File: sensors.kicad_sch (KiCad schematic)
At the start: 17 parts, among them Q2 TEMT6000X01, U6 BME280, U7 MAX4466EXK

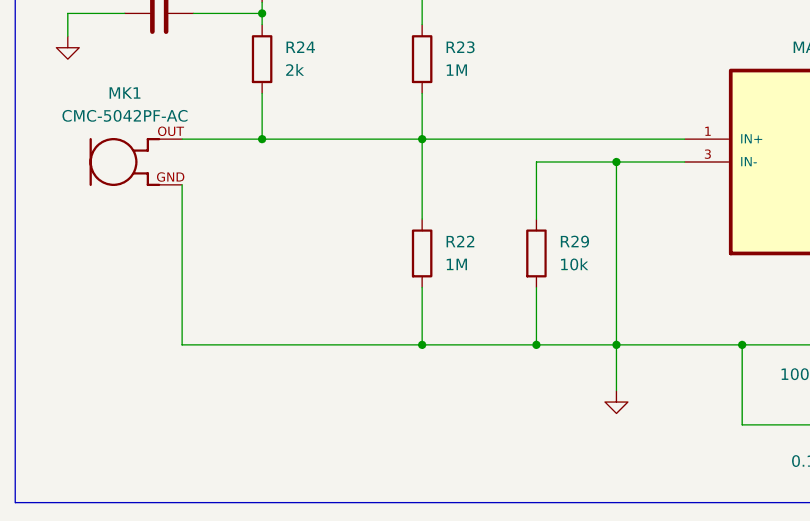
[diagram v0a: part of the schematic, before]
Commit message: wip layout 1
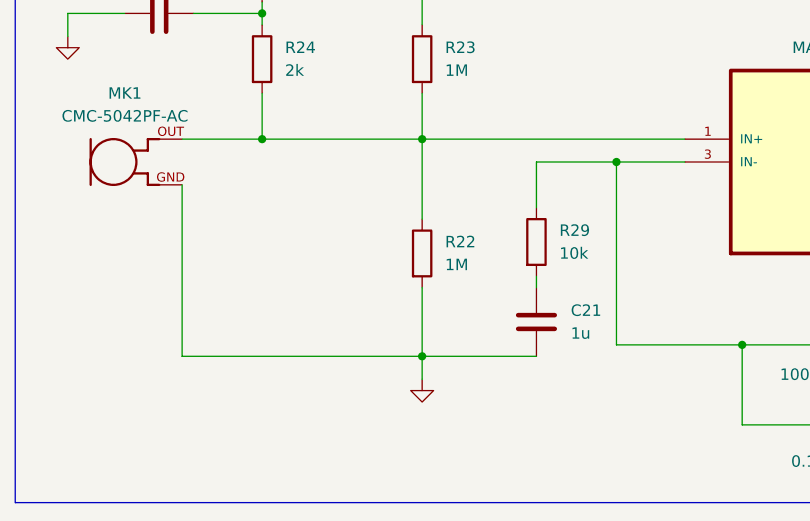
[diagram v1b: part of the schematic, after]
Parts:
- added C21: 1u, Capacitor_SMD:C_0805_2012Metric, symbol Device:C
- MK1: footprint CMC-5042PF-AC:CUI_CMC-5042PF-AC -> esp32 footprints:CUI_CMC-5042PF-AC
- Q2: footprint TEMT6000X01:TRANS_TEMT6000X01 -> esp32 footprints:TRANS_TEMT6000X01
- U6: footprint BME280:PSON65P250X250X100-8N -> esp32 footprints:PSON65P250X250X100-8N
- U7: footprint MAX4466EXK:SOT65P210X110-5N -> esp32 footprints:SOT65P210X110-5N
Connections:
- net GND: now also C21.2; no longer C19.2, R29.1, R29.2, R30.1, U7.3 (IN-)
- new net: C19.2, R29.1, R30.1, U7.3 (IN-)
- new net: C21.1, R29.2
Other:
- moved on the sheet: R29
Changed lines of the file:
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@@
 	)
 	(junction
-		(at 189.23 142.24)
+		(at 198.12 121.92)
 		(diameter 0)
 		(color 0 0 0 0)
 	)
 	(junction
-		(at 198.12 121.92)
+		(at 176.53 143.51)
 		(diameter 0)
 		(color 0 0 0 0)
@@
 	)
 	(junction
-		(at 176.53 142.24)
-		(diameter 0)
-		(color 0 0 0 0)
-	)
-	(junction
 		(at 255.27 114.3)
 		(diameter 0)
@@
 	)
 	(junction
-		(at 198.12 142.24)
-		(diameter 0)
-		(color 0 0 0 0)
-	)
-	(junction
 		(at 176.53 119.38)
 		(diameter 0)
@@
 	(wire
 		(pts
+			(xy 189.23 134.62) (xy 189.23 135.89)
+		)
+		(stroke
+			(width 0)
+			(type default)
+		)
+	)
+	(wire
+		(pts
 			(xy 26.67 63.5) (xy 35.56 63.5)
 		)
@@
 	(wire
 		(pts
-			(xy 189.23 142.24) (xy 198.12 142.24)
+			(xy 176.53 143.51) (xy 189.23 143.51)
 		)
 		(stroke
@@
 	(wire
 		(pts
-			(xy 189.23 135.89) (xy 189.23 142.24)
-		)
-		(stroke
-			(width 0)
-			(type default)
-		)
-	)
-	(wire
-		(pts
-			(xy 149.86 124.46) (xy 149.86 142.24)
+			(xy 149.86 124.46) (xy 149.86 143.51)
 		)
 		(stroke
@@
 	(wire
 		(pts
-			(xy 198.12 142.24) (xy 198.12 147.32)
+			(xy 255.27 114.3) (xy 255.27 110.49)
 		)
 		(stroke
@@
 	(wire
 		(pts
-			(xy 255.27 114.3) (xy 255.27 110.49)
+			(xy 105.41 69.85) (xy 105.41 73.66)
 		)
 		(stroke
@@
 	(wire
 		(pts
-			(xy 105.41 69.85) (xy 105.41 73.66)
+			(xy 176.53 143.51) (xy 176.53 146.05)
 		)
 		(stroke
@@
 	(wire
 		(pts
-			(xy 189.23 128.27) (xy 189.23 121.92)
+			(xy 189.23 127) (xy 189.23 121.92)
 		)
 		(stroke
@@
 	(wire
 		(pts
-			(xy 176.53 142.24) (xy 189.23 142.24)
-		)
-		(stroke
-			(width 0)
-			(type default)
-		)
-	)
-	(wire
-		(pts
 			(xy 158.75 105.41) (xy 158.75 106.68)
 		)
@@
 	(wire
 		(pts
-			(xy 149.86 142.24) (xy 176.53 142.24)
+			(xy 149.86 143.51) (xy 176.53 143.51)
 		)
 		(stroke
@@
 	(wire
 		(pts
-			(xy 176.53 135.89) (xy 176.53 142.24)
+			(xy 176.53 135.89) (xy 176.53 143.51)
 		)
 		(stroke
@@
 			)
 		)
-		(property "Footprint" "MAX4466EXK:SOT65P210X110-5N"
+		(property "Footprint" "esp32 footprints:SOT65P210X110-5N"
 			(at 223.52 121.92 0)
 			(effects
@@
 			)
 		)
-		(property "Footprint" "TEMT6000X01:TRANS_TEMT6000X01"
+		(property "Footprint" "esp32 footprints:TRANS_TEMT6000X01"
 			(at 149.86 54.61 0)
 			(effects
@@
 	(symbol
 		(lib_id "Device:R")
-		(at 189.23 132.08 0)
+		(at 189.23 130.81 0)
 		(unit 1)
 		(exclude_from_sim no)
@@
 		(fields_autoplaced yes)
 		(property "Reference" "R29"
-			(at 191.77 130.8099 0)
+			(at 191.77 129.5399 0)
 			(effects
 				(font
@@
 		)
 		(property "Value" "10k"
-			(at 191.77 133.3499 0)
+			(at 191.77 132.0799 0)
 			(effects
 				(font
@@
 		)
 		(property "Footprint" "Resistor_SMD:R_0805_2012Metric"
-			(at 187.452 132.08 90)
+			(at 187.452 130.81 90)
 			(effects
 				(font
@@
 		)
 		(property "Datasheet" "~"
-			(at 189.23 132.08 0)
+			(at 189.23 130.81 0)
 			(effects
 				(font
@@
 		)
 		(property "Description" "Resistor"
-			(at 189.23 132.08 0)
+			(at 189.23 130.81 0)
 			(effects
 				(font
@@
 			)
 		)
-		(property "Footprint" "BME280:PSON65P250X250X100-8N"
+		(property "Footprint" "esp32 footprints:PSON65P250X250X100-8N"
 			(at 83.82 59.69 0)
 			(effects
@@
 			)
 		)
-		(property "Footprint" "CMC-5042PF-AC:CUI_CMC-5042PF-AC"
+		(property "Footprint" "esp32 footprints:CUI_CMC-5042PF-AC"
 			(at 142.24 121.92 0)
 			(effects
@@
 	)
 	(symbol
+		(lib_id "Device:C")
+		(at 189.23 139.7 0)
+		(unit 1)
+		(exclude_from_sim no)
+		(in_bom yes)
+		(on_board yes)
+		(dnp no)
+		(fields_autoplaced yes)
+		(property "Reference" "C21"
+			(at 193.04 138.4299 0)
+			(effects
+				(font
+					(size 1.27 1.27)
+				)
+				(justify left)
+			)
+		)
+		(property "Value" "1u"
+			(at 193.04 140.9699 0)
+			(effects
+				(font
+					(size 1.27 1.27)
+				)
+				(justify left)
+			)
+		)
+		(property "Footprint" "Capacitor_SMD:C_0805_2012Metric"
+			(at 190.1952 143.51 0)
+			(effects
+				(font
+					(size 1.27 1.27)
+				)
+				(hide yes)
+			)
+		)
+		(property "Datasheet" "~"
+			(at 189.23 139.7 0)
+			(effects
+				(font
+					(size 1.27 1.27)
+				)
+				(hide yes)
+			)
+		)
+		(property "Description" "Unpolarized capacitor"
+			(at 189.23 139.7 0)
+			(effects
+				(font
+					(size 1.27 1.27)
+				)
+				(hide yes)
+			)
+		)
+		(pin "1"
+		)
+		(pin "2"
+		)
+		(instances
+			(project ""
+				(path "/0c27022e-f7a1-45ca-b269-a51d4ff975b0/989a141a-e25e-45c3-9987-b10e8b0a6e30/032a409b-9df2-444c-a15c-8ddac32e6f43"
+					(reference "C21")
+					(unit 1)
+				)
+			)
+		)
+	)
+	(symbol
 		(lib_id "power:+3V3")
 		(at 167.64 90.17 0)
@@
 	(symbol
 		(lib_id "power:GND")
-		(at 198.12 147.32 0)
+		(at 176.53 146.05 0)
 		(unit 1)
 		(exclude_from_sim no)
@@
 		(fields_autoplaced yes)
 		(property "Reference" "#PWR044"
-			(at 198.12 153.67 0)
+			(at 176.53 152.4 0)
 			(effects
 				(font
@@
 		)
 		(property "Value" "GND"
-			(at 198.12 152.4 0)
+			(at 176.53 151.13 0)
 			(effects
 				(font
@@
 		)
 		(property "Footprint" ""
-			(at 198.12 147.32 0)
+			(at 176.53 146.05 0)
 			(effects
 				(font
@@
 		)
 		(property "Datasheet" ""
-			(at 198.12 147.32 0)
+			(at 176.53 146.05 0)
 			(effects
 				(font
@@
 		)
 		(property "Description" "Power symbol creates a global label with name \"GND\" , ground"
-			(at 198.12 147.32 0)
+			(at 176.53 146.05 0)
 			(effects
 				(font

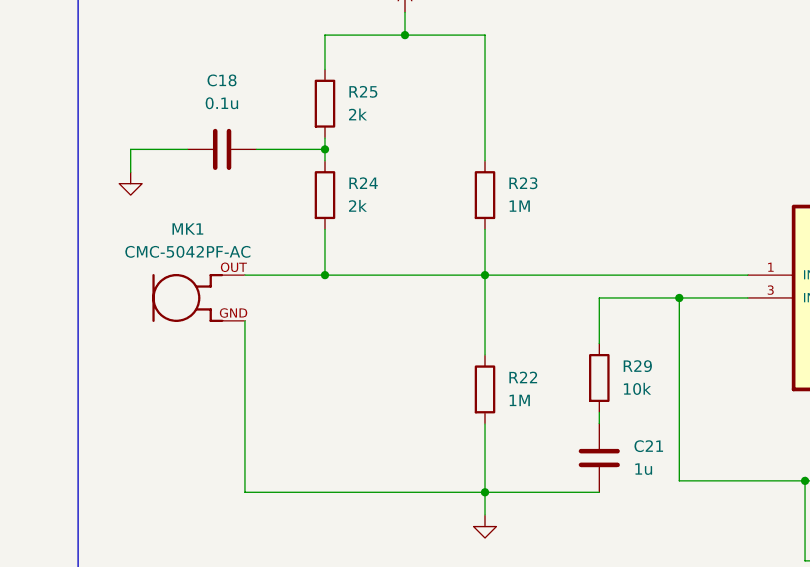
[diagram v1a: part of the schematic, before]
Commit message: placement complete
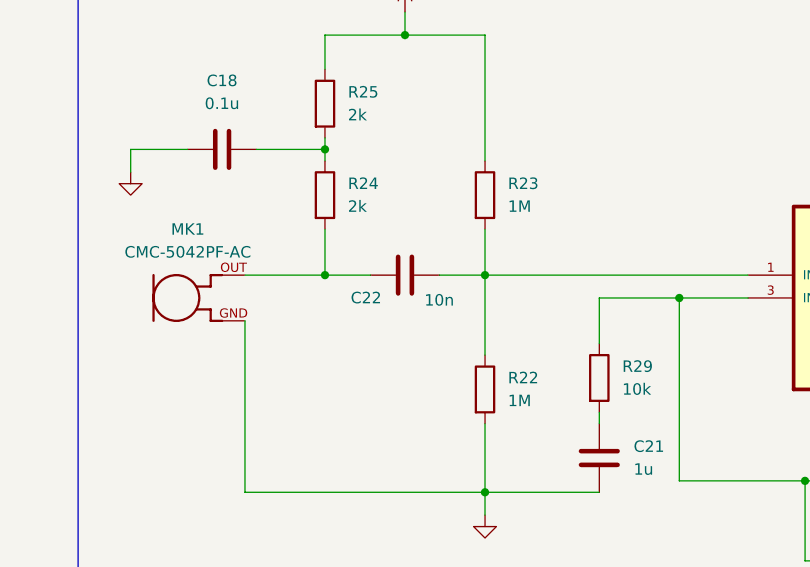
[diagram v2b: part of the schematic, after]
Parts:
- added C22: 10n, Capacitor_SMD:C_0805_2012Metric, symbol Device:C
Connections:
- net at R22.1, R23.2, U7.1 (IN+): now also C22.2; no longer MK1.OUT, R24.2
- new net: C22.1, MK1.OUT, R24.2
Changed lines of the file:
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@@
+	)
+	(junction
+		(at 158.75 119.38)
+		(diameter 0)
+		(color 0 0 0 0)
 	)
 	(junction
@@
 	)
 	(junction
-		(at 158.75 119.38)
-		(diameter 0)
-		(color 0 0 0 0)
-	)
-	(junction
 		(at 105.41 49.53)
 		(diameter 0)
@@
 	(wire
 		(pts
-			(xy 158.75 119.38) (xy 176.53 119.38)
-		)
-		(stroke
-			(width 0)
-			(type default)
-		)
-	)
-	(wire
-		(pts
 			(xy 45.72 53.34) (xy 45.72 50.8)
 		)
@@
 	(wire
 		(pts
+			(xy 171.45 119.38) (xy 176.53 119.38)
+		)
+		(stroke
+			(width 0)
+			(type default)
+		)
+	)
+	(wire
+		(pts
 			(xy 158.75 105.41) (xy 158.75 106.68)
 		)
@@
 		(pts
 			(xy 105.41 52.07) (xy 105.41 49.53)
+		)
+		(stroke
+			(width 0)
+			(type default)
+		)
+	)
+	(wire
+		(pts
+			(xy 158.75 119.38) (xy 163.83 119.38)
 		)
 		(stroke
@@
 					(unit 1)
 				)
+			)
+		)
+	)
+	(symbol
+		(lib_id "Device:C")
+		(at 167.64 119.38 90)
+		(unit 1)
+		(exclude_from_sim no)
+		(in_bom yes)
+		(on_board yes)
+		(dnp no)
+		(property "Reference" "C22"
+			(at 163.322 121.92 90)
+			(effects
+				(font
+					(size 1.27 1.27)
+				)
+			)
+		)
+		(property "Value" "10n"
+			(at 171.45 122.174 90)
+			(effects
+				(font
+					(size 1.27 1.27)
+				)
+			)
+		)
+		(property "Footprint" "Capacitor_SMD:C_0805_2012Metric"
+			(at 171.45 118.4148 0)
+			(effects
+				(font
+					(size 1.27 1.27)
+				)
+				(hide yes)
+			)
+		)
+		(property "Datasheet" "~"
+			(at 167.64 119.38 0)
+			(effects
+				(font
+					(size 1.27 1.27)
+				)
+				(hide yes)
+			)
+		)
+		(property "Description" "Unpolarized capacitor"
+			(at 167.64 119.38 0)
+			(effects
+				(font
+					(size 1.27 1.27)
+				)
+				(hide yes)
+			)
+		)
+		(pin "1"
+		)
+		(pin "2"
+		)
+		(instances
+			(project ""
+				(path "/0c27022e-f7a1-45ca-b269-a51d4ff975b0/989a141a-e25e-45c3-9987-b10e8b0a6e30/032a409b-9df2-444c-a15c-8ddac32e6f43"
+					(reference "C22")
+					(unit 1)
+				)
